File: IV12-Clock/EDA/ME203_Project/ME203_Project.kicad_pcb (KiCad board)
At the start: 2 copper layers, 76.2 x 54.4 mm, 65 parts, among them J1 Conn_01x12, J11 Conn_01x02, J2 Conn_01x05, J3 Conn_01x06, J4 Conn_01x02, J5 Conn_01x02, J6 Conn_01x07, Q1 AO4294, SW1 SW_Push, SW2 SW_Push, T1 WE-FLEX_ER11_5, U1 LM3478SOIC8, U2 CD40109, U3 TPS82140SILR, U4 ESP32-WROOM, U5 BMP280

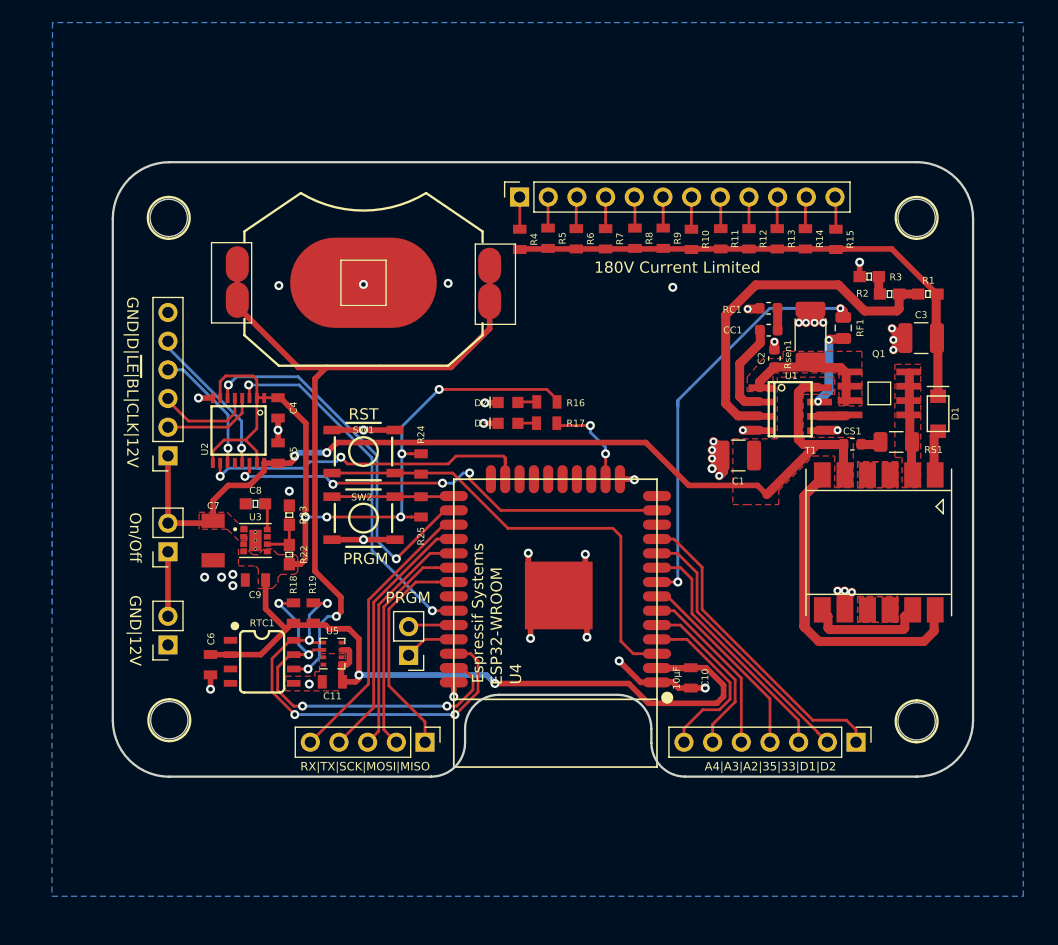
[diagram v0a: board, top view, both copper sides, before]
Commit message: Code KWS, working on actual time.
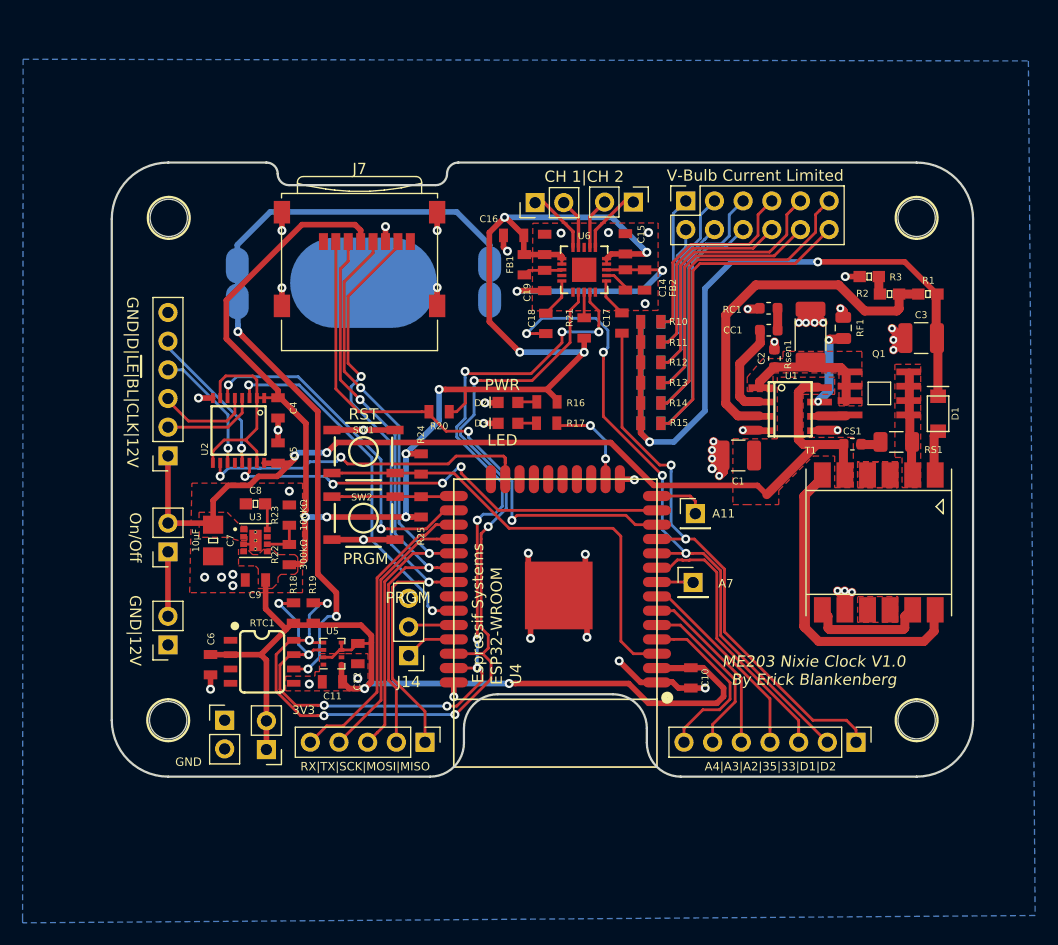
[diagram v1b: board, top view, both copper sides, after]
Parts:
- added C12: 0.1µF, 0805, F.Cu at (94.5, 77.6)
- added C13: 0.1µF, 0805, F.Cu at (111.0, 41.4)
- added C14: 0.1µF, 0805, F.Cu at (118.2, 44.5)
- added C15: 10µF, 0805, F.Cu at (118.2, 41.3)
- added C16: 10µF, 0805, F.Cu at (108.3, 40.5)
- added C17: 1µF, 0805, F.Cu at (117.9, 48.3)
- added C18: 1µF, 0805, F.Cu at (111.2, 48.4)
- added C19: 0.1µF, 0805, F.Cu at (111.0, 44.5)
- added FB1: Ferrite_Bead, 0805, F.Cu at (109.2, 43.1)
- added FB2: Ferrite_Bead, 0805, F.Cu at (119.9, 44.5)
- added J10: Conn_01x01, Connector_PinHeader_2.54mm:PinHeader_1x01_P2.54mm_Vertical, F.Cu at (124.2, 71.3)
- added J12: Conn_01x01, Connector_PinHeader_2.54mm:PinHeader_1x01_P2.54mm_Vertical, F.Cu at (124.4, 65.2)
- added J13: Conn_01x02, Connector_PinHeader_2.54mm:PinHeader_1x02_P2.54mm_Vertical, F.Cu at (82.7, 83.5)
- added J14: Conn_01x03, Connector_PinHeader_2.54mm:PinHeader_1x03_P2.54mm_Vertical, F.Cu at (99.0, 77.8)
- added J7: Micro_SD_Card, Connector_Card:microSD_HC_Wuerth_693072010801, F.Cu at (94.7, 42.6)
- added J8: Conn_01x02, Connector_PinHeader_2.54mm:PinHeader_1x02_P2.54mm_Vertical, F.Cu at (118.9, 37.6)
- added J9: Conn_01x02, Connector_PinHeader_2.54mm:PinHeader_1x02_P2.54mm_Vertical, F.Cu at (110.2, 37.6)
- added R20: 100kΩ, 0805, F.Cu at (101.7, 56.2)
- added R21: 100KΩ, 0805, F.Cu at (114.5, 48.8)
- added U6: TPA2016D2RTJR, QFN50P400X400X80-21N, F.Cu at (114.5, 43.6)
- BT1, R4, R5, R6, R7, R8, R9: moved to B.Cu
- C11, C4, C5: value 1.0µF -> 0.1µF
- C7: footprint 1210 -> 1206
- CS1: value 380pF -> 360pF
- J1: footprint Connector_PinSocket_2.54mm:PinSocket_1x12_P2.54mm_Vertical -> Connector_PinSocket_2.54mm:PinSocket_2x06_P2.54mm_Vertical
- R22, R23: footprint 0603 -> 0805
- moved R15 23.1 mm to (120.5, 57.2), turned to 180 degrees
- moved R14 20.0 mm to (120.5, 55.4), turned to 180 degrees
- moved R13 17.0 mm to (120.5, 53.6), turned to 180 degrees
- moved R9 16.4 mm to (120.5, 57.2), turned to 180 degrees
- moved J11 15.1 mm to (86.4, 86.1)
- moved J1 14.7 mm to (123.5, 37.5)
- moved R8 14.7 mm to (120.5, 55.4), turned to 180 degrees
- moved R12 14.0 mm to (120.5, 51.8), turned to 180 degrees
- moved R4 13.7 mm to (120.5, 48.2), turned to 180 degrees
- moved R7 13.4 mm to (120.5, 53.6), turned to 180 degrees
- moved R5 12.9 mm to (120.5, 50.0), turned to 180 degrees
- moved R6 12.8 mm to (120.5, 51.8), turned to 180 degrees
- moved R11 11.0 mm to (120.5, 50.0), turned to 180 degrees
- moved R10 8.14 mm to (120.5, 48.2), turned to 180 degrees
- moved H1 0.10 mm to (77.7, 83.5)
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- renumbered H1 to H3
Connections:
- net /ESP32/A0-DAC2 renamed /DAC2
- net /ESP32/A1-DAC1 renamed /DAC1
- net /ESP32/A5-D4 renamed /ESP32/A5-T0-D4
- net /ESP32/A6-D14 renamed /ESP32/A6-T6-D14
- net /ESP32/A9-D33 renamed /ESP32/A9-T8-D33
- net /MCU_RTC/SCL renamed /MCU_Audio/SCL
- net /MCU_RTC/SDA renamed /MCU_Audio/SDA
- J11 pad 1: /ESP32/TXD0 -> +3V3
- J11 pad 2: /ESP32/RXD0 -> +3V3
- RF1 pad 1: /ESP32/A7-D32 -> GND
- U4 pad 12: /ESP32/A10-D27 -> /ESP32/SD-Select
- U4 pad 14: /ESP32/A11-D12 -> /ESP32/A11-T5-D12
- U4 pad 8: /ESP32/A7-D32 -> /ESP32/A7-T9-D32
- U5 pad 2: Net-(U5-Pad2) -> +3V3
- U5 pad 5: Net-(U5-Pad5) -> +3V3
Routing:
- net +3V3: track 147.5 -> 241.9 mm, vias 7 -> 11
- net /ESP32/SD-Select: track 0.00 -> 49.3 mm, vias 0 -> 2
- net /MCU_Audio/SDA: track 36.4 -> 85.1 mm, vias 4 -> 10
- net /MCU_Audio/SCL: track 39.8 -> 83.4 mm, vias 4 -> 6
- net /ESP32/A7-D32: track 37.1 -> 0.00 mm, vias 2 -> 0
- net /ESP32/MISO-D19: track 19.9 -> 56.3 mm, vias 0 -> 2
- net /DAC1: track 24.0 -> 58.2 mm, vias 0 -> 4
- net /ESP32/MOSI-D18: track 20.1 -> 53.1 mm, vias 0 -> 2
- net /ESP32/SCK-D5: track 21.1 -> 53.8 mm, vias 0 -> 2
- net Net-(J1-Pad11): track 2.88 -> 29.1 mm
- net Net-(J1-Pad12): track 2.93 -> 28.7 mm
- net /Nixie_PSU/180V: track 47.9 -> 70.8 mm, vias 0 -> 2
- net /DAC2: track 27.9 -> 50.1 mm, vias 0 -> 2
- net AGND: track 0.00 -> 21.1 mm, vias 0 -> 2
- net Net-(J1-Pad9): track 2.85 -> 23.7 mm
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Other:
- board size 76.2 x 54.4 mm -> 76.3 x 54.4 mm
- net class Default: clearance 0.2 -> 0.09
- rule trace_clearance: 0.2 -> 0.09
- board text added: "3V3"
- board text added: "A11"
- board text added: "A7"
- board text added: "CH 1|CH 2"
- board text added: "GND"
- board text added: "LED"
- board text added: "ME203 Nixie Clock V1.0 By Erick Blankenberg"
- board text added: "PWR"
- board text added: "V-Bulb Current Limited"
- board text removed: "180V Current Limited"
